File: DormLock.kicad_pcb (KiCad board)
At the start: 2 copper layers, 84.9 x 81.7 mm, 66 parts, among them J1 Conn_02x03_Odd_Even, J10 Conn_02x03_Odd_Even, J2 Conn_01x05, J4 Conn_01x03, J5 Conn_01x02, J6 Conn_01x15, J7 Conn_01x15, J8 Conn_01x08, J9 USB_C_Receptacle, Q1 Q_NPN_BEC, Q2 Q_PMOS_GSD, Q3 Q_PMOS_GSD, SW1 SW_Push, U1 SPX1117M3-L-3-3/TR, U2 SY8105, U3 STM32F030CCTx, U4 LM321

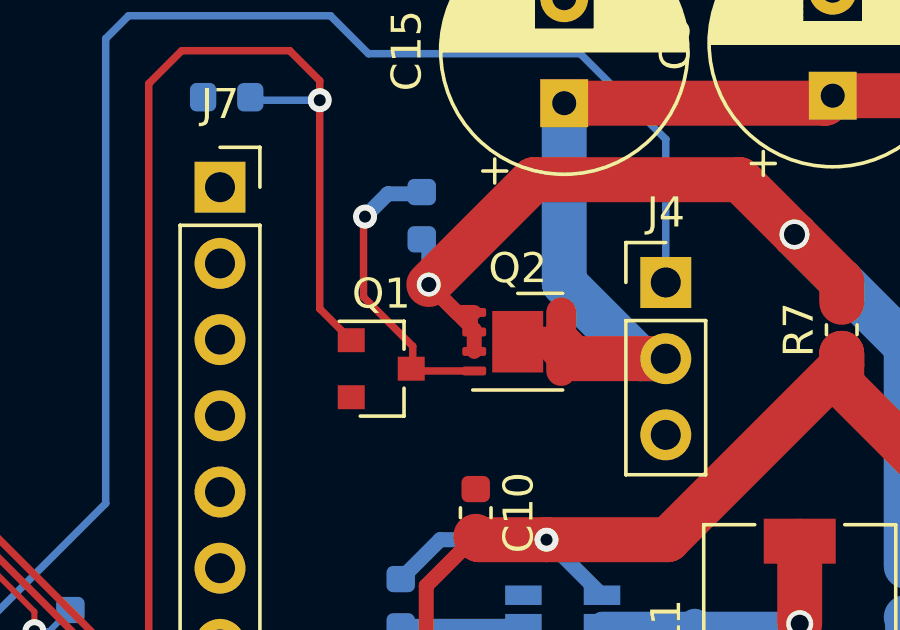
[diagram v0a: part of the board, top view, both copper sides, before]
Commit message: V2.0
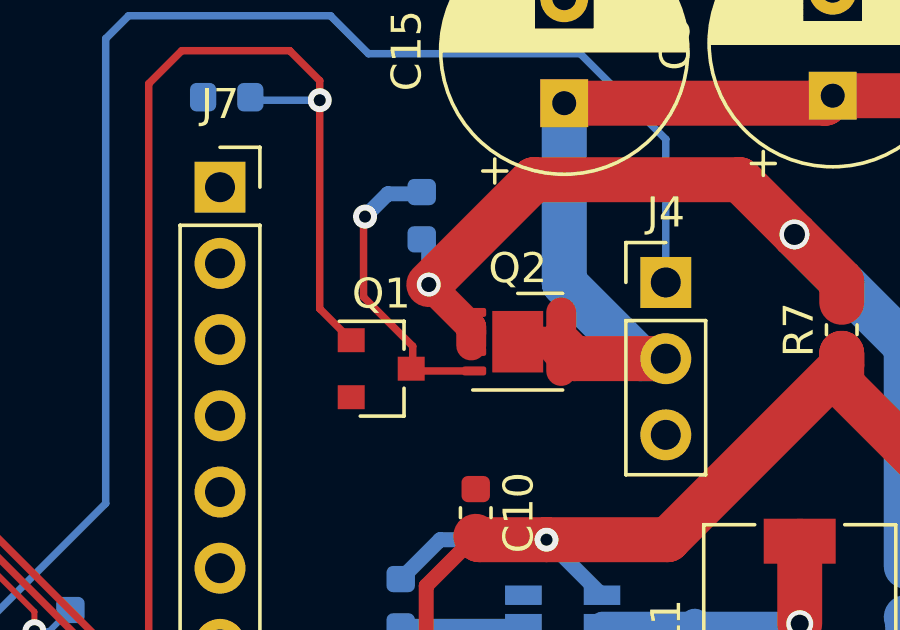
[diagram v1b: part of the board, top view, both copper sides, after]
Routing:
- net Vdrive: track 37.6 -> 34.1 mm
